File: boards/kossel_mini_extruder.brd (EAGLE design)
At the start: 76.9 x 69 mm, 26 parts

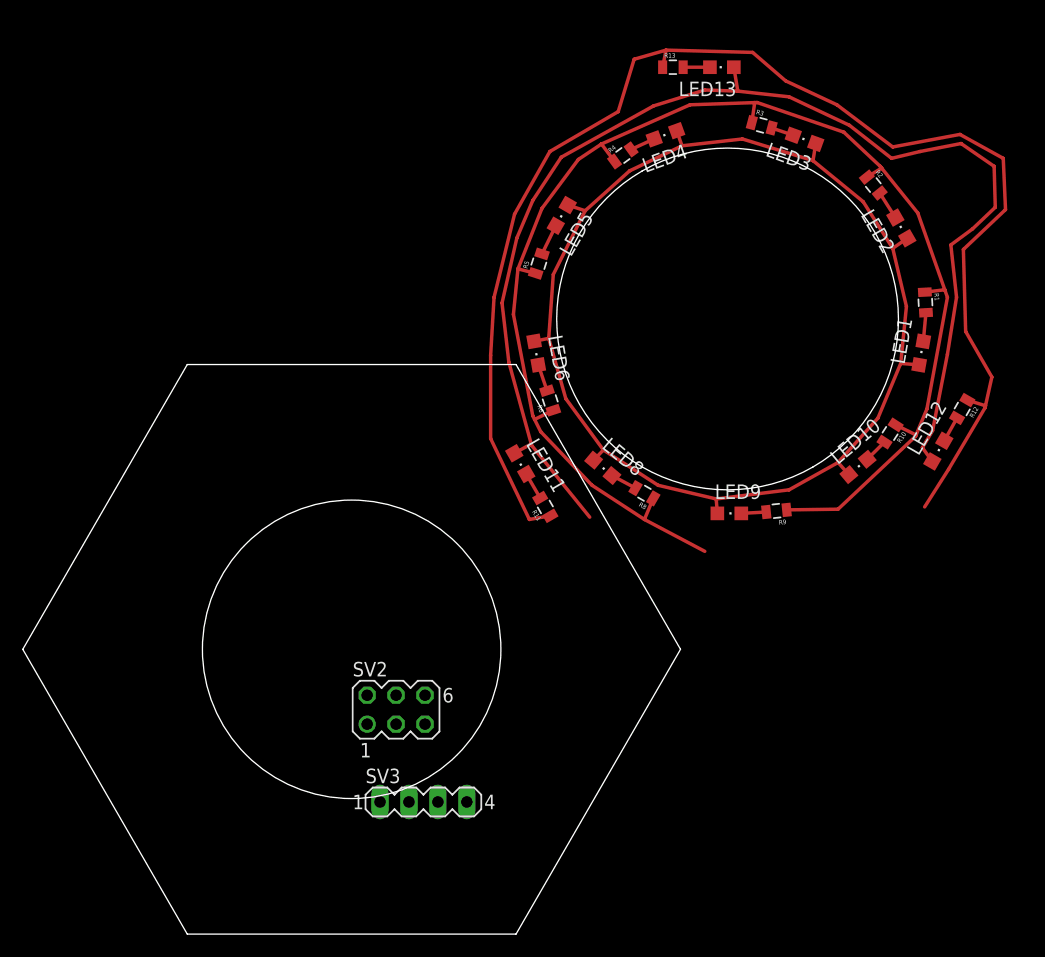
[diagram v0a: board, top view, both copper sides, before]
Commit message: still grinding on board
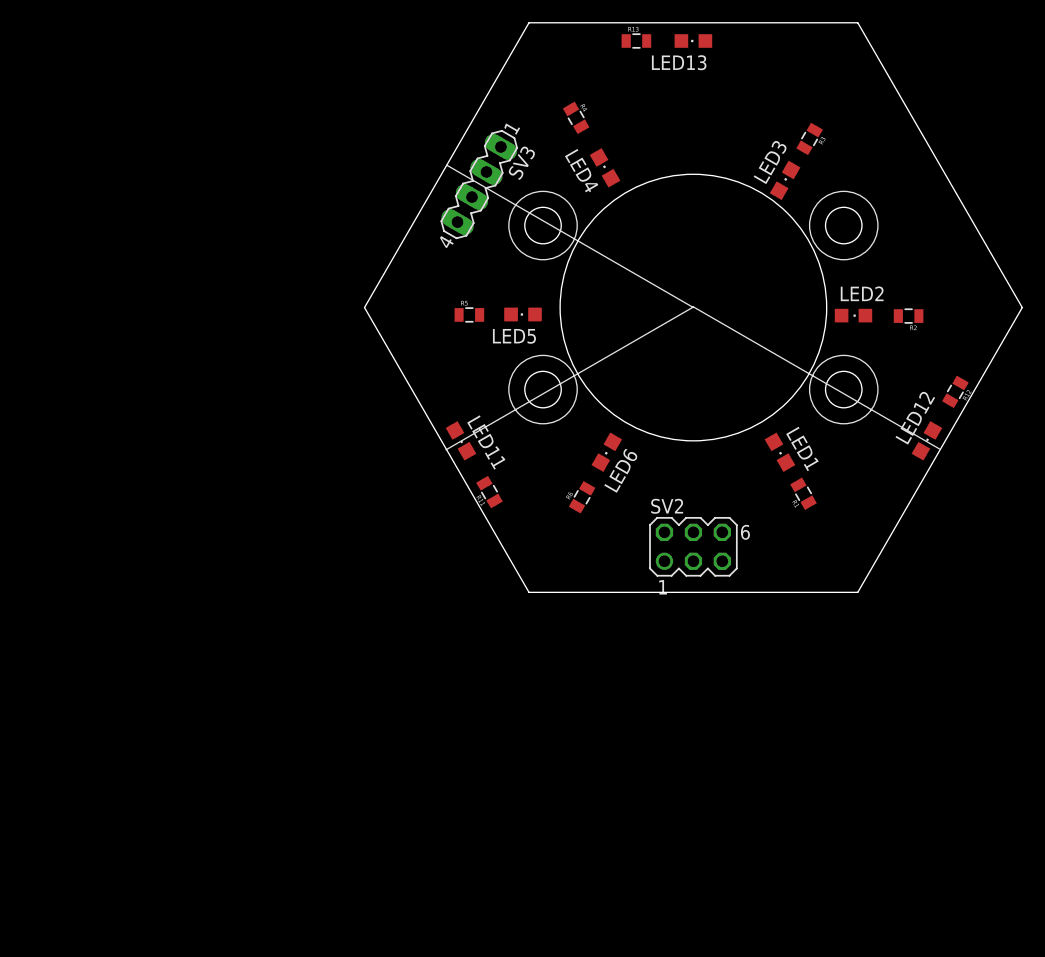
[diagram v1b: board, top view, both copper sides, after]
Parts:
- removed LED10, LED8, LED9: (no value), SparkFun-LED:CHIPLED_0805
- removed R10, R8, R9: (no value), SparkFun-Passives:0805
- moved SV3 54.4 mm to (11.2, 40.8), turned to 240 degrees
- moved SV2 29.8 mm to (30.0, 9.00)
- moved R1 19.9 mm to (39.7, 13.7), turned to 120 degrees
- moved LED1 15.1 mm to (37.6, 17.3), turned to 300 degrees
- moved R2 11.9 mm to (48.9, 29.3), turned to 180 degrees
- moved LED6 10.7 mm to (22.4, 17.3), turned to 240 degrees
- moved LED5 9.34 mm to (15.0, 29.4), turned to 180 degrees
- moved R6 8.95 mm to (20.2, 13.3), turned to 60 degrees
- moved LED2 8.77 mm to (44.1, 29.3), turned to 0 degrees
- moved R5 7.58 mm to (10.3, 29.4), turned to 0 degrees
- moved LED4 6.04 mm to (22.2, 42.3), turned to 120 degrees
- moved LED11 5.57 mm to (9.60, 18.3)
- moved R4 5.26 mm to (19.7, 46.7), turned to 300 degrees
- moved R11 5.07 mm to (12.1, 13.8)
- moved R3 4.37 mm to (40.2, 44.8), turned to 240 degrees
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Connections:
- removed net N$13: LED9.C, R9.2
- removed net N$14: LED10.C, R10.2
- removed net N$9: LED8.C, R8.2
- net GND: no longer R10.1, R8.1, R9.1
- net VCC: no longer LED10.A, LED8.A, LED9.A
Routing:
- net GND: track 126.9 -> 0.00 mm
- net HOT_12V: track 121.1 -> 0.00 mm
- net VCC: track 111.7 -> 0.00 mm
- net HOT_SIG: track 108.9 -> 0.00 mm
- net N$5: track 2.75 -> 0.00 mm
- net N$2: track 2.55 -> 0.00 mm
- net N$1: track 2.53 -> 0.00 mm
- net N$16: track 2.44 -> 0.00 mm
- net N$6: track 2.39 -> 0.00 mm
- net N$18: track 2.35 -> 0.00 mm
- net N$9: track 2.35 -> 0.00 mm
- net N$17: track 2.30 -> 0.00 mm
- net N$4: track 2.23 -> 0.00 mm
- net N$13: track 2.20 -> 0.00 mm
- net N$14: track 2.14 -> 0.00 mm
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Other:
- board size 76.9 x 69 mm -> 57.7 x 50 mm
